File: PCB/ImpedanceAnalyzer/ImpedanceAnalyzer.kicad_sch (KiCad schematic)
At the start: 0 parts

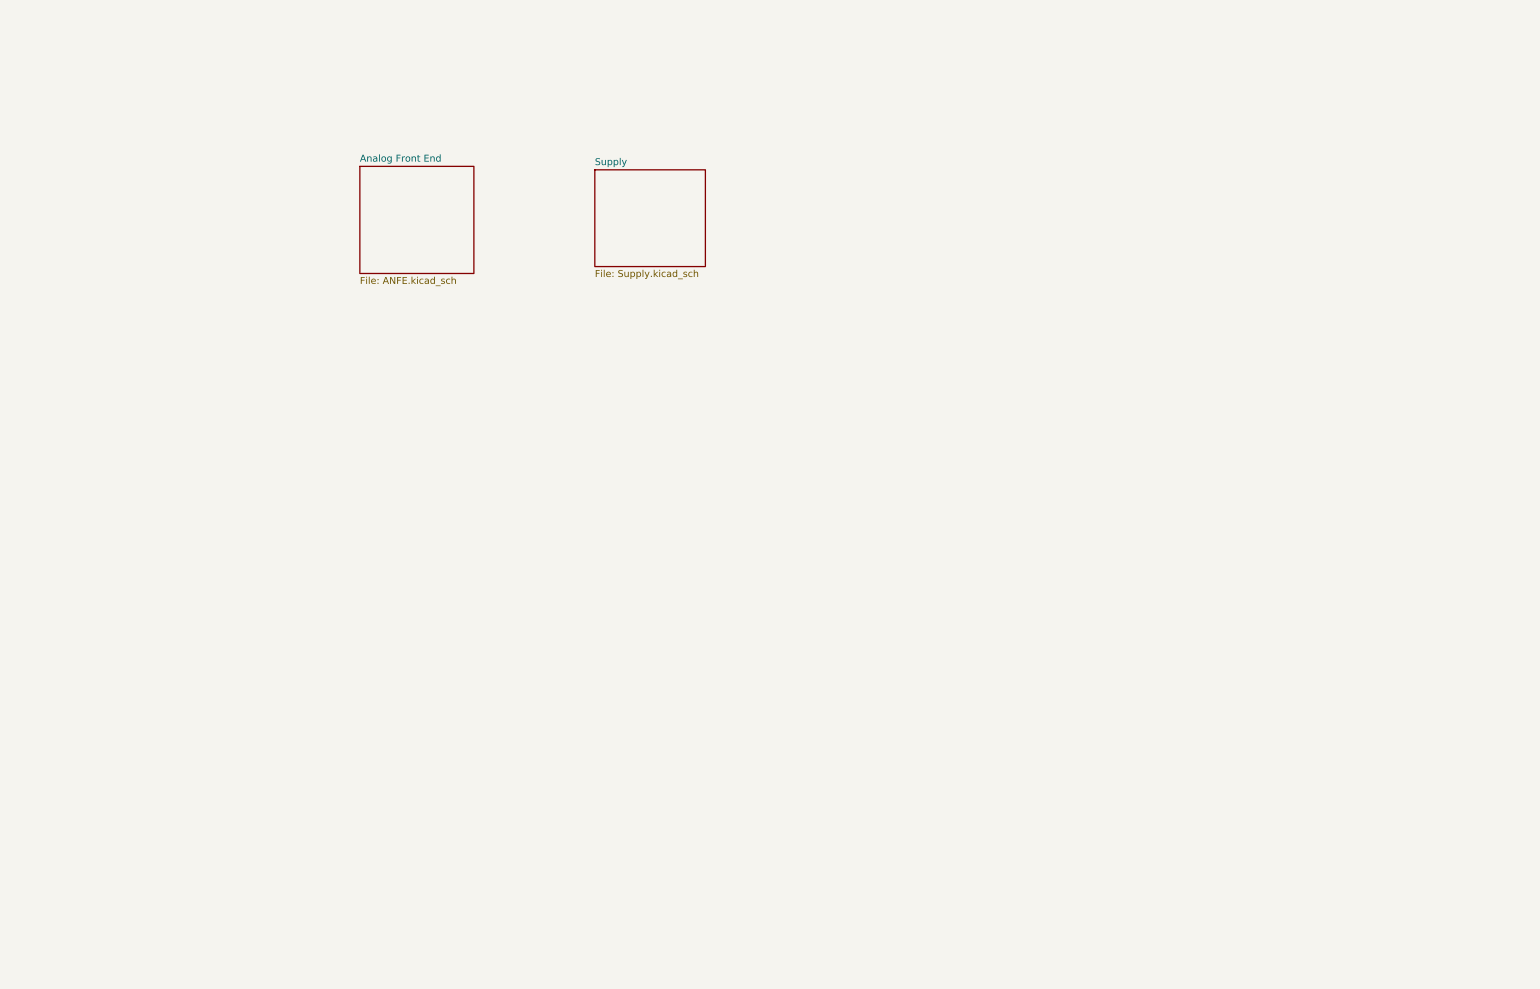
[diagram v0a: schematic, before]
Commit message: schematic v1
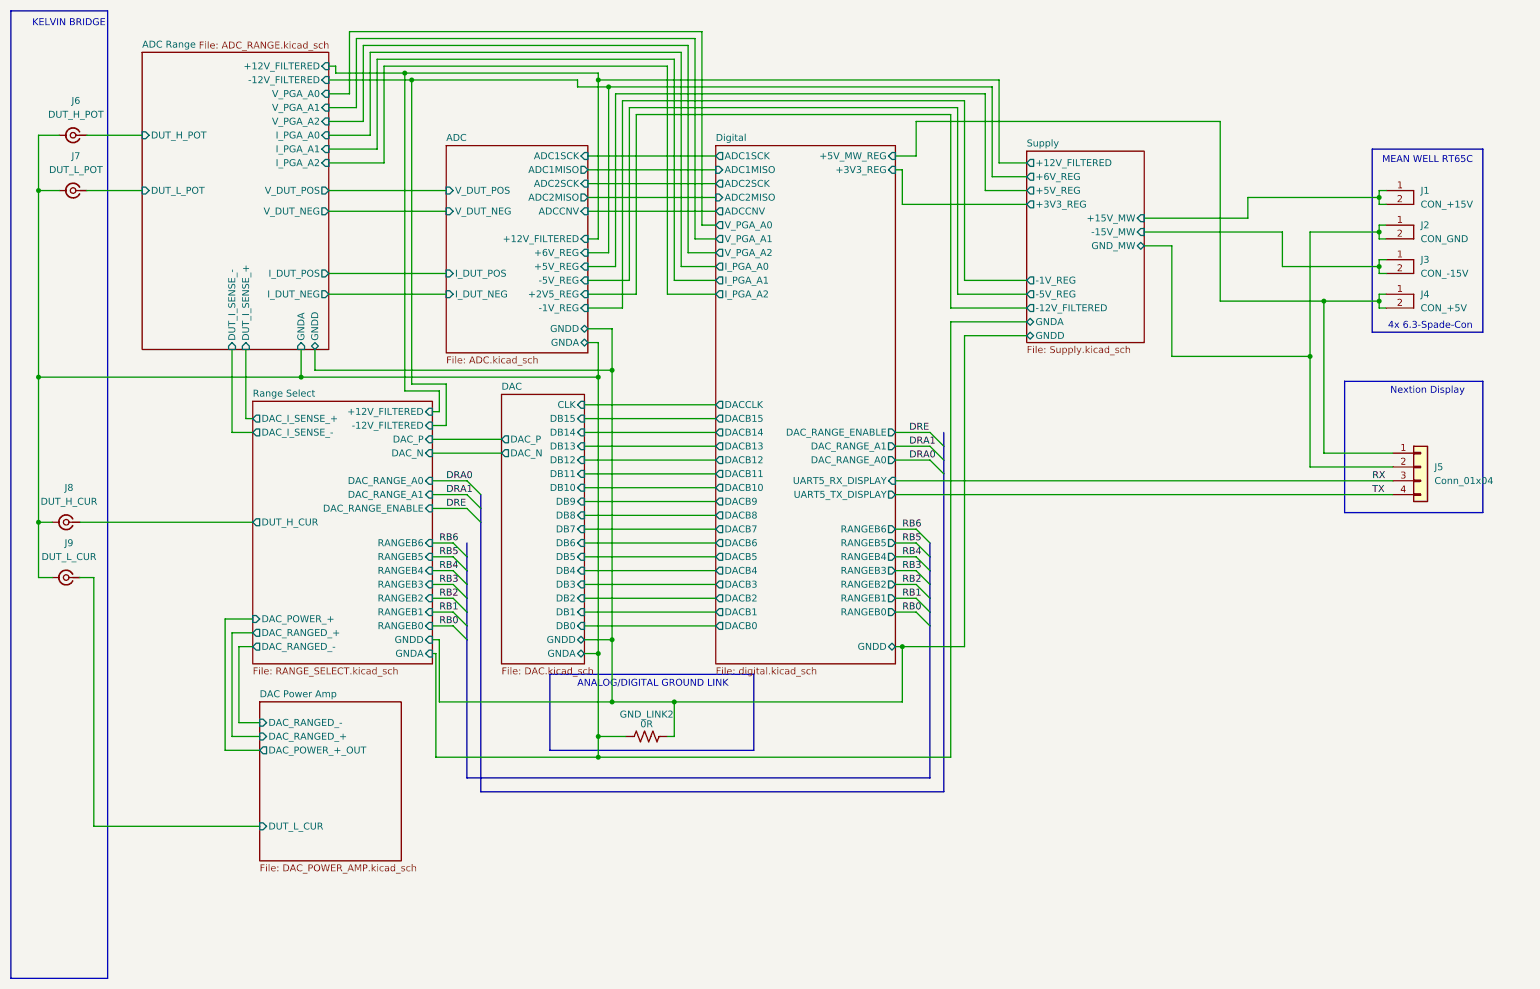
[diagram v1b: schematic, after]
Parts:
- added GND_LINK2: 0R, symbol Device:R_US
- added J1: CON_+15V, symbol JRIX Connector:6.3-Spade-Con
- added J2: CON_GND, symbol JRIX Connector:6.3-Spade-Con
- added J3: CON_-15V, symbol JRIX Connector:6.3-Spade-Con
- added J4: CON_+5V, symbol JRIX Connector:6.3-Spade-Con
- added J5: Conn_01x04, symbol Connector_Generic:Conn_01x04
- added J6: DUT_H_POT, symbol Connector:Conn_Coaxial_Small
- added J7: DUT_L_POT, symbol Connector:Conn_Coaxial_Small
- added J8: DUT_H_CUR, symbol Connector:Conn_Coaxial_Small
- added J9: DUT_L_CUR, symbol Connector:Conn_Coaxial_Small
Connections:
- new net ADC Range/DUT_H_POT: J6.1 (In)
- new net ADC Range/DUT_L_POT: J7.1 (In)
- new net ADC Range/GNDA: GND_LINK2.1, J6.2 (Ext), J7.2 (Ext), J8.2 (Ext), J9.2 (Ext)
- new net ADC Range/GNDD: GND_LINK2.2
- new net DAC Power Amp/DUT_L_CUR: J9.1 (In)
- new net Digital/+5V_MW_REG: J4.1, J4.2, J5.1 (Pin_1)
- new net RX: J5.3 (Pin_3)
- new net Range Select/DUT_H_CUR: J8.1 (In)
- new net Supply/+15V_MW: J1.1, J1.2
- new net Supply/-15V_MW: J3.1, J3.2
- new net Supply/GND_MW: J2.1, J2.2, J5.2 (Pin_2)
- new net TX: J5.4 (Pin_4)
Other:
- sheet Analog Front End renamed ADC
- added sheet ADC Range (ADC_RANGE.kicad_sch)
- added sheet DAC (DAC.kicad_sch)
- added sheet DAC Power Amp (DAC_POWER_AMP.kicad_sch)
- added sheet Digital (digital.kicad_sch)
- added sheet Range Select (RANGE_SELECT.kicad_sch)
- sheet ADC: file ANFE.kicad_sch -> ADC.kicad_sch
- sheet ADC ports: added +12V_FILTERED, +2V5_REG, +5V_REG, +6V_REG, -1V_REG, -5V_REG, ADC1MISO, ADC1SCK, ADC2MISO, ADC2SCK, ADCCNV, GNDA, GNDD, I_DUT_NEG, I_DUT_POS, V_DUT_NEG, V_DUT_POS; removed none
- sheet Supply ports: added +12V_FILTERED, +15V_MW, +3V3_REG, +5V_REG, +6V_REG, -12V_FILTERED, -15V_MW, -1V_REG, -5V_REG, GNDA, GNDD, GND_MW; removed none
- note added: "4x 6.3-Spade-Con"
- note added: "ANALOG/DIGITAL GROUND LINK"
- note added: "KELVIN BRIDGE"
- note added: "MEAN WELL RT65C"
- note added: "Nextion Display"

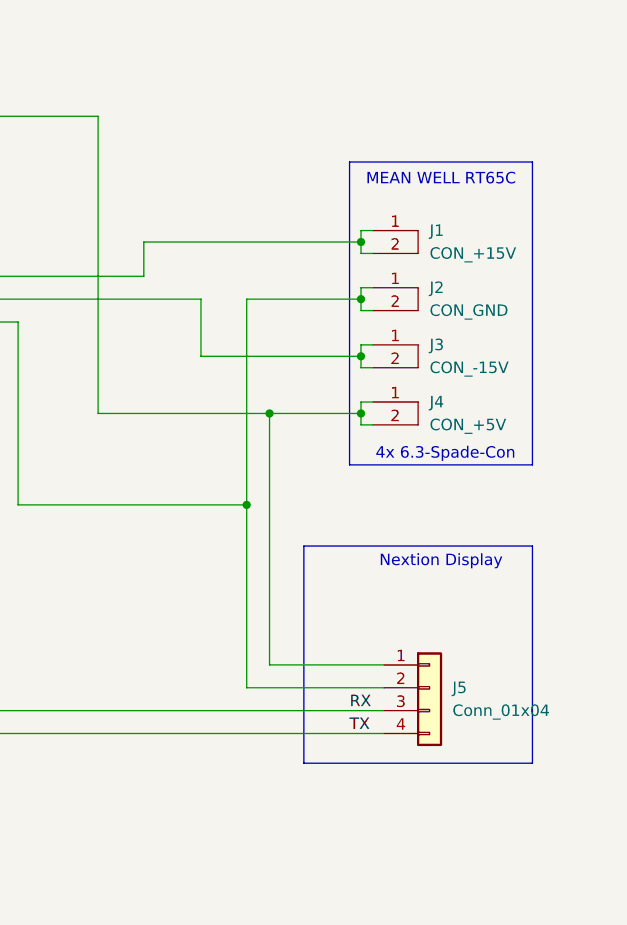
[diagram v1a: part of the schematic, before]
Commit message: ready for pcb
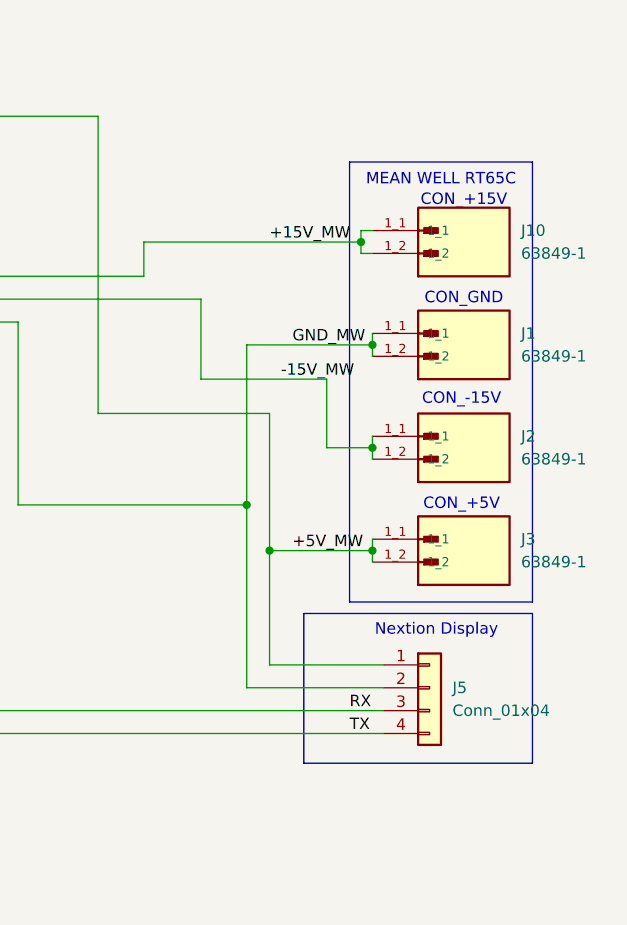
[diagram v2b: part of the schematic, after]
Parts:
- removed J1: CON_+15V, symbol JRIX Connector:6.3-Spade-Con
- removed J2: CON_GND, symbol JRIX Connector:6.3-Spade-Con
- removed J3: CON_-15V, symbol JRIX Connector:6.3-Spade-Con
- removed J4: CON_+5V, symbol JRIX Connector:6.3-Spade-Con
- added J1, J10, J2, J3: 63849-1, JRIX FASTON Connectors Footprints:TE_63849-1, symbol JRIX FASTON Connector:63849-1
- GND_LINK2: footprint (none) -> JRIX Resistor SMD:Resistor SMD - 2818
- J5: footprint (none) -> Connector_JST:JST_XH_B4B-XH-A_1x04_P2.50mm_Vertical
- J6, J7, J8, J9: footprint (none) -> Connector_Coaxial:BNC_TEConnectivity_1478204_Vertical
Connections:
- net Digital/+5V_MW_REG renamed +5V_MW
- net +5V_MW: now also J3.1_1, J3.1_2
- net Supply/GND_MW renamed GND_MW
- net GND_MW: now also J1.1_1, J1.1_2
- new net +15V_MW: J10.1_1, J10.1_2
- new net -15V_MW: J2.1_1, J2.1_2
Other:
- note added: "CON_+15V"
- note added: "CON_+5V"
- note added: "CON_-15V"
- note added: "CON_GND"
- note removed: "4x 6.3-Spade-Con"
